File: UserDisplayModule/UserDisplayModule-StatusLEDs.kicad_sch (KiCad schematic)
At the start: 15 parts, among them U1 74HC595

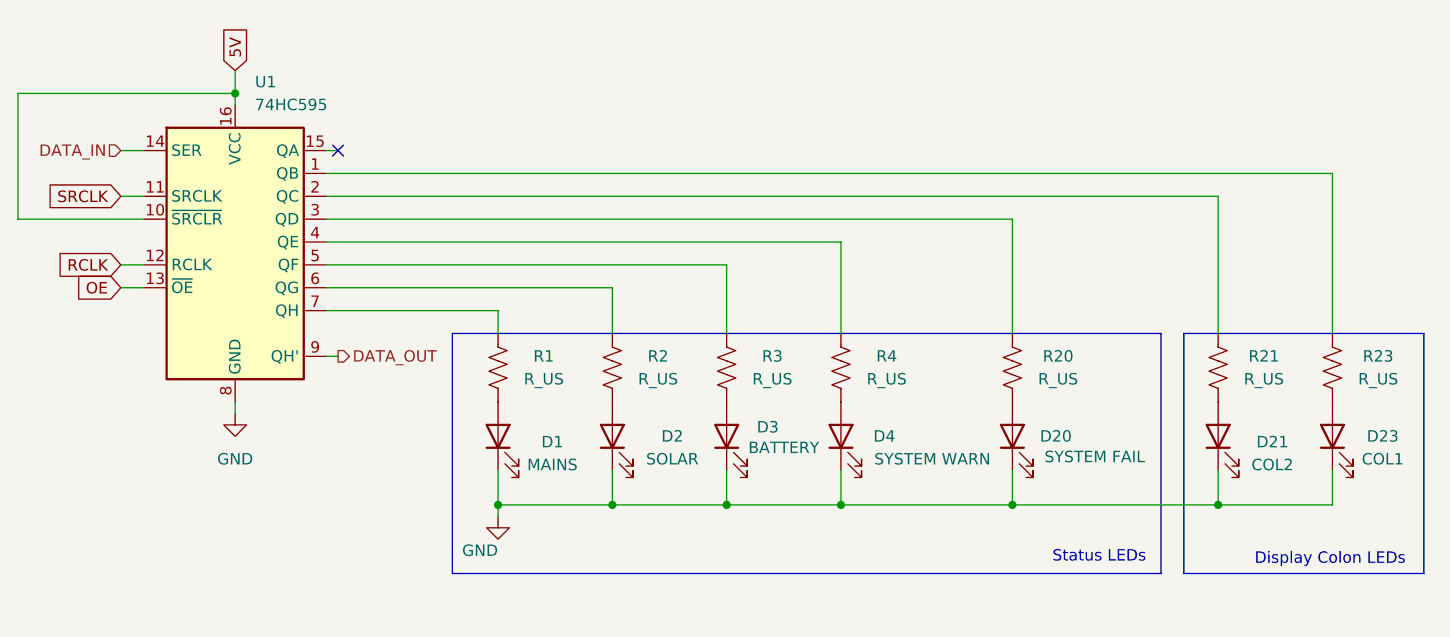
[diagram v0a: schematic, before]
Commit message: doubled LEDs + started PCB
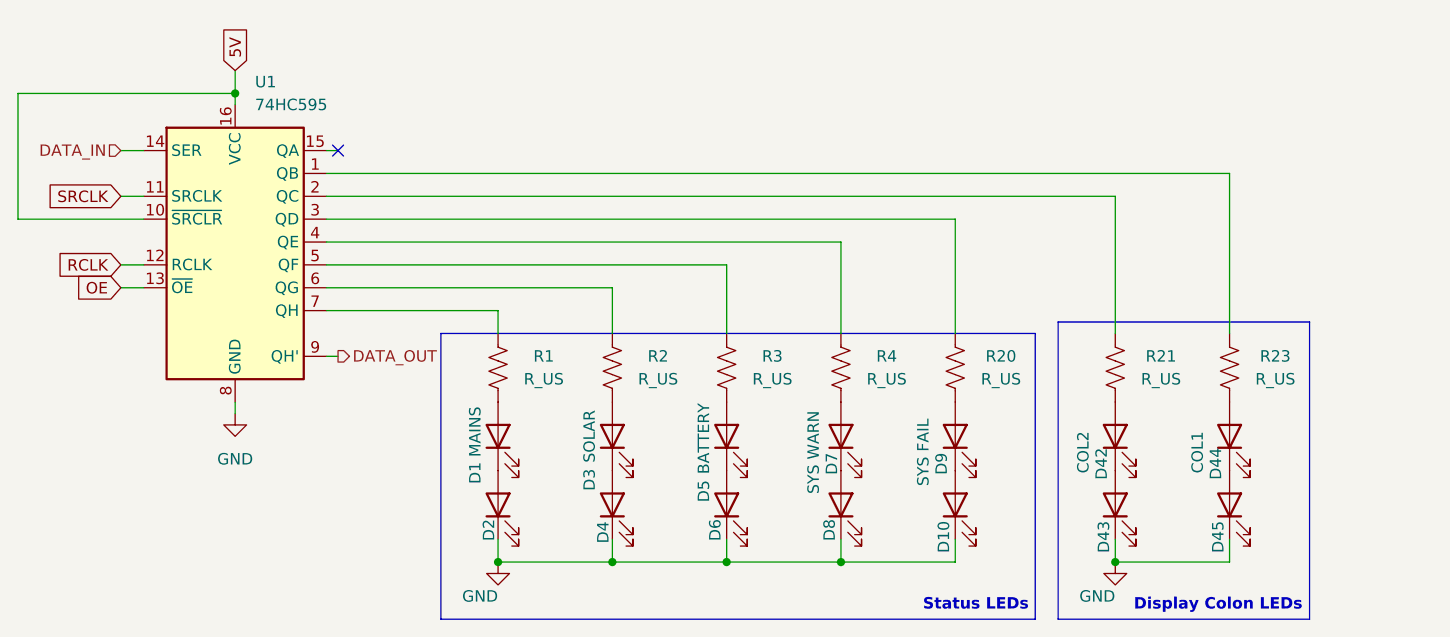
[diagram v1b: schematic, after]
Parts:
- removed D20: SYSTEM FAIL, symbol Device:LED
- removed D21: COL2, symbol Device:LED
- removed D23: COL1, symbol Device:LED
- removed D4: SYSTEM WARN, symbol Device:LED
- added D10, D43, D45: BAT3, LED_SMD:LED_0805_2012Metric, symbol Device:LED
- added D2: MAINS, LED_SMD:LED_0805_2012Metric, symbol Device:LED
- added D42: COL2, LED_SMD:LED_0805_2012Metric, symbol Device:LED
- added D44: COL1, LED_SMD:LED_0805_2012Metric, symbol Device:LED
- added D5: BATTERY, LED_SMD:LED_0805_2012Metric, symbol Device:LED
- added D6: BAT7, LED_SMD:LED_0805_2012Metric, symbol Device:LED
- added D7: SYS WARN, LED_SMD:LED_0805_2012Metric, symbol Device:LED
- added D8: BAT5, LED_SMD:LED_0805_2012Metric, symbol Device:LED
- added D9: SYS FAIL, LED_SMD:LED_0805_2012Metric, symbol Device:LED
- D1: footprint (none) -> LED_SMD:LED_0805_2012Metric
- D3: renamed from D2; footprint (none) -> LED_SMD:LED_0805_2012Metric
- D4: renamed from D3; footprint (none) -> LED_SMD:LED_0805_2012Metric
- R1, R2, R20, R21, R23, R3, R4: footprint (none) -> Resistor_SMD:R_0805_2012Metric
- U1: footprint (none) -> ImportedFootprints:CD74HC595E
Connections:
- net GND: now also D10.1 (K), D2.1 (K), D43.1 (K), D45.1 (K), D6.1 (K), D8.1 (K); no longer D1.1 (K), D3.1 (K)
- net at R21.2: now also D42.2 (A)
- net at R23.2: now also D44.2 (A)
- net at R3.2: now also D5.2 (A); no longer D4.2 (A)
- net at R20.2: now also D9.2 (A)
- net at R4.2: now also D7.2 (A)
- new net: D42.1 (K), D43.2 (A)
- new net: D44.1 (K), D45.2 (A)
- new net: D7.1 (K), D8.2 (A)
- new net: D1.1 (K), D2.2 (A)
- new net: D3.1 (K), D4.2 (A)
- new net: D10.2 (A), D9.1 (K)
- new net: D5.1 (K), D6.2 (A)
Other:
- moved on the sheet: D4, R20, R21, R23

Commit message: started routing (help)
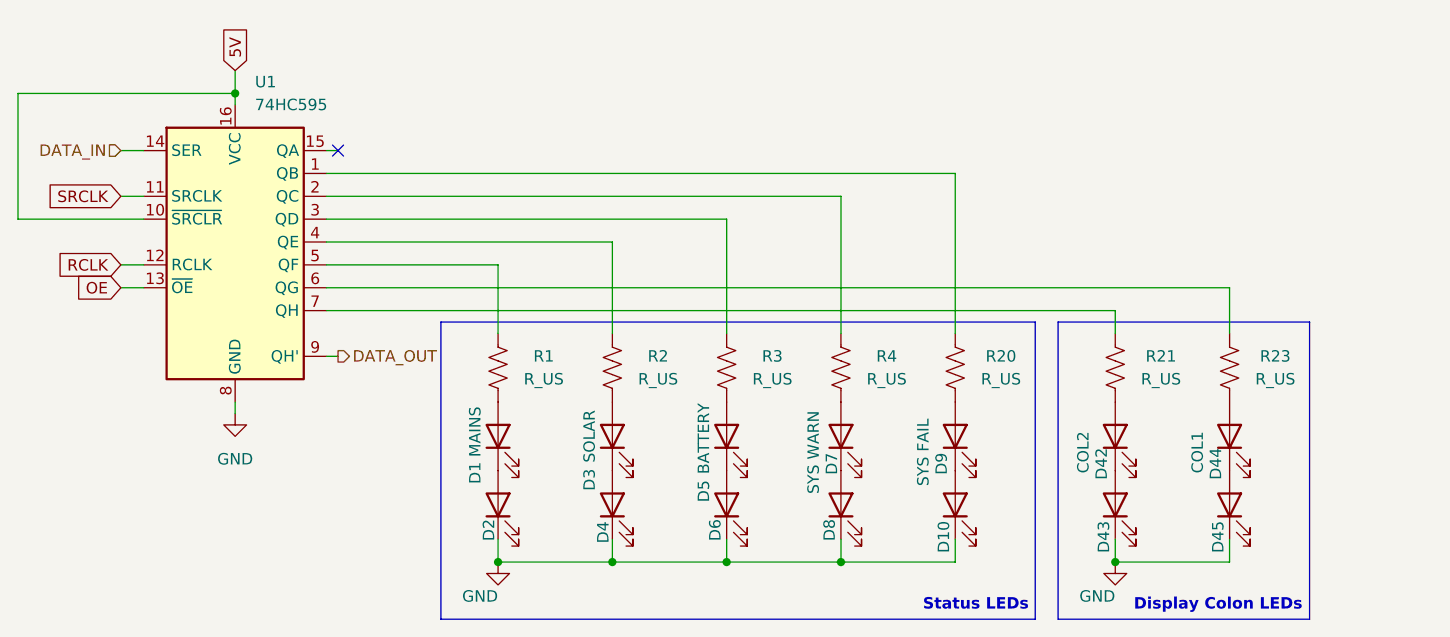
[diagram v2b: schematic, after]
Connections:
- net at R23.1: now also U1.6 (QG); no longer U1.1 (QB)
- net at R1.1: now also U1.5 (QF); no longer U1.7 (QH)
- net at R3.1: now also U1.3 (QD); no longer U1.5 (QF)
- net at R21.1: now also U1.7 (QH); no longer U1.2 (QC)
- net at R20.1: now also U1.1 (QB); no longer U1.3 (QD)
- net at R2.1: now also U1.4 (QE); no longer U1.6 (QG)
- net at R4.1: now also U1.2 (QC); no longer U1.4 (QE)
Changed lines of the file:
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@@
-	(wire
-		(pts
-			(xy 100.33 83.82) (xy 157.48 83.82)
-		)
-		(stroke
-			(width 0)
-			(type default)
-		)
-	)
 	(wire
 		(pts
@@
 	(wire
 		(pts
+			(xy 100.33 88.9) (xy 200.66 88.9)
+		)
+		(stroke
+			(width 0)
+			(type default)
+		)
+	)
+	(wire
+		(pts
+			(xy 100.33 78.74) (xy 157.48 78.74)
+		)
+		(stroke
+			(width 0)
+			(type default)
+		)
+	)
+	(wire
+		(pts
 			(xy 119.38 119.38) (xy 132.08 119.38)
 		)
@@
 	(wire
 		(pts
+			(xy 100.33 76.2) (xy 170.18 76.2)
+		)
+		(stroke
+			(width 0)
+			(type default)
+		)
+	)
+	(wire
+		(pts
 			(xy 77.47 86.36) (xy 80.01 86.36)
 		)
@@
 	(wire
 		(pts
-			(xy 157.48 83.82) (xy 157.48 93.98)
-		)
-		(stroke
-			(width 0)
-			(type default)
-		)
-	)
-	(wire
-		(pts
-			(xy 100.33 76.2) (xy 200.66 76.2)
+			(xy 100.33 91.44) (xy 187.96 91.44)
 		)
 		(stroke
@@
 	(wire
 		(pts
-			(xy 100.33 81.28) (xy 170.18 81.28)
-		)
-		(stroke
-			(width 0)
-			(type default)
-		)
-	)
-	(wire
-		(pts
-			(xy 144.78 86.36) (xy 144.78 93.98)
-		)
-		(stroke
-			(width 0)
-			(type default)
-		)
-	)
-	(wire
-		(pts
-			(xy 119.38 91.44) (xy 119.38 93.98)
+			(xy 132.08 83.82) (xy 132.08 93.98)
+		)
+		(stroke
+			(width 0)
+			(type default)
+		)
+	)
+	(wire
+		(pts
+			(xy 187.96 91.44) (xy 187.96 93.98)
 		)
 		(stroke
@@
 	(wire
 		(pts
-			(xy 100.33 86.36) (xy 144.78 86.36)
-		)
-		(stroke
-			(width 0)
-			(type default)
-		)
-	)
-	(wire
-		(pts
 			(xy 157.48 119.38) (xy 170.18 119.38)
 		)
@@
 	(wire
 		(pts
-			(xy 100.33 78.74) (xy 187.96 78.74)
-		)
-		(stroke
-			(width 0)
-			(type default)
-		)
-	)
-	(wire
-		(pts
 			(xy 100.33 96.52) (xy 101.6 96.52)
 		)
@@
 	(wire
 		(pts
+			(xy 144.78 81.28) (xy 144.78 93.98)
+		)
+		(stroke
+			(width 0)
+			(type default)
+		)
+	)
+	(wire
+		(pts
 			(xy 77.47 73.66) (xy 80.01 73.66)
 		)
@@
 	(wire
 		(pts
-			(xy 170.18 81.28) (xy 170.18 93.98)
+			(xy 119.38 86.36) (xy 119.38 93.98)
 		)
 		(stroke
@@
 	(wire
 		(pts
-			(xy 100.33 91.44) (xy 119.38 91.44)
-		)
-		(stroke
-			(width 0)
-			(type default)
-		)
-	)
-	(wire
-		(pts
 			(xy 77.47 78.74) (xy 80.01 78.74)
 		)
@@
 	(wire
 		(pts
-			(xy 132.08 88.9) (xy 132.08 93.98)
-		)
-		(stroke
-			(width 0)
-			(type default)
-		)
-	)
-	(wire
-		(pts
-			(xy 187.96 78.74) (xy 187.96 93.98)
-		)
-		(stroke
-			(width 0)
-			(type default)
-		)
-	)
-	(wire
-		(pts
-			(xy 200.66 76.2) (xy 200.66 93.98)
+			(xy 100.33 81.28) (xy 144.78 81.28)
+		)
+		(stroke
+			(width 0)
+			(type default)
+		)
+	)
+	(wire
+		(pts
+			(xy 100.33 83.82) (xy 132.08 83.82)
+		)
+		(stroke
+			(width 0)
+			(type default)
+		)
+	)
+	(wire
+		(pts
+			(xy 157.48 78.74) (xy 157.48 93.98)
+		)
+		(stroke
+			(width 0)
+			(type default)
+		)
+	)
+	(wire
+		(pts
+			(xy 200.66 88.9) (xy 200.66 93.98)
 		)
 		(stroke
@@
 	(wire
 		(pts
-			(xy 100.33 88.9) (xy 132.08 88.9)
+			(xy 170.18 76.2) (xy 170.18 93.98)
 		)
 		(stroke
@@
 		)
 	)
+	(wire
+		(pts
+			(xy 100.33 86.36) (xy 119.38 86.36)
+		)
+		(stroke
+			(width 0)
+			(type default)
+		)
+	)
 	(rectangle
-		(start 113.03 93.98)
+		(start 113.03 92.71)
 		(end 179.07 125.73)
 		(stroke
